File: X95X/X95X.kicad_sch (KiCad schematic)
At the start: 21 parts, among them J1 AVR-ISP-6, J2 USB_C_Receptacle_USB2.0, SW92 SW_Push, U1 ATmega32U4-A, Y1 Crystal_GND24_Small

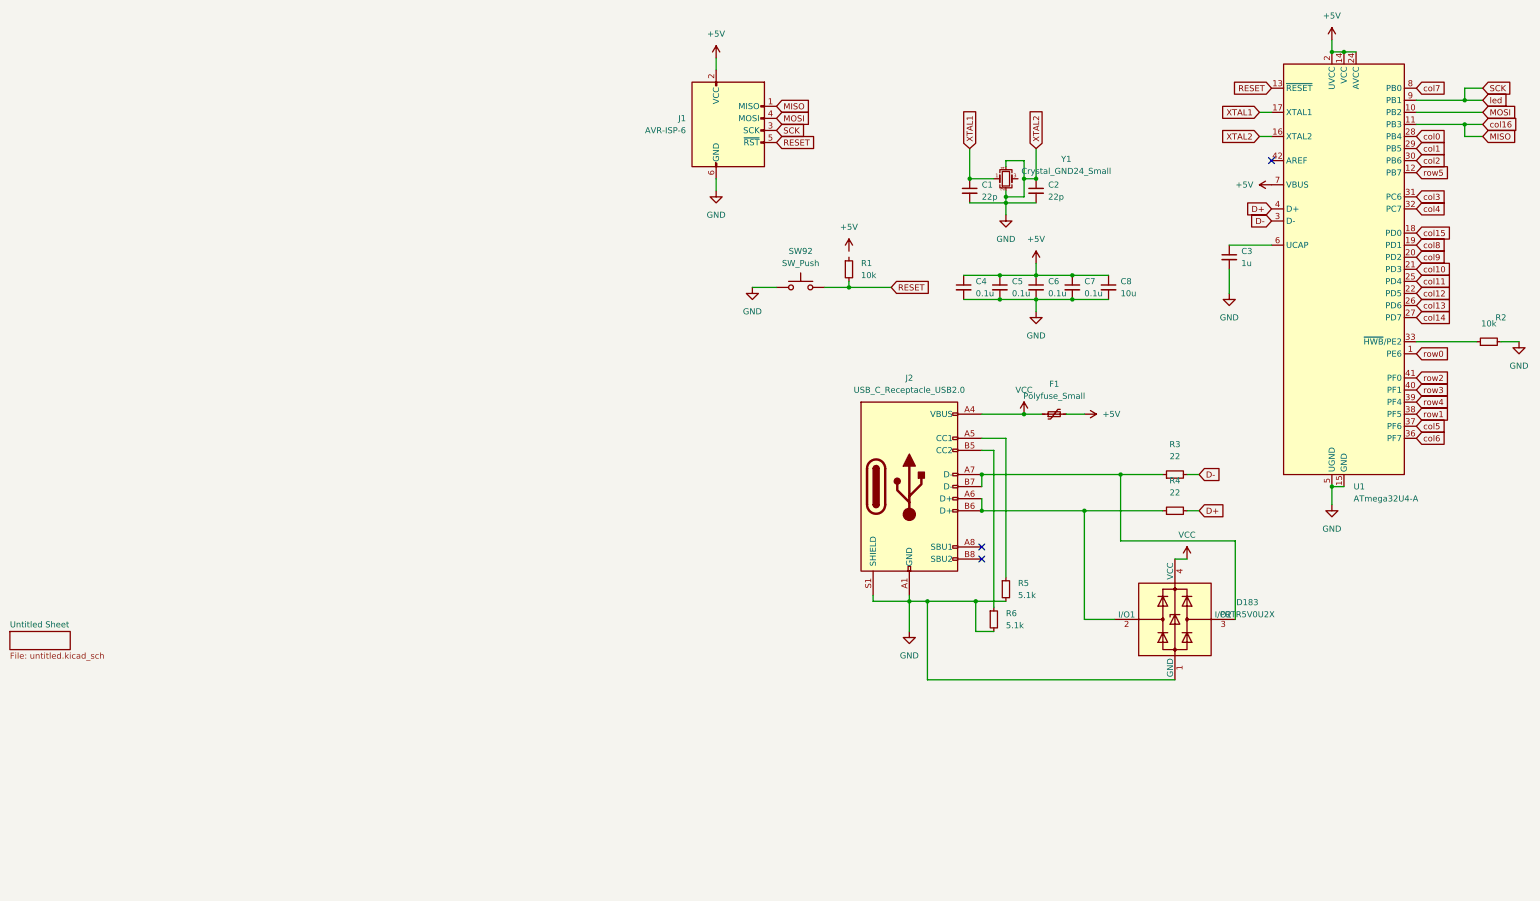
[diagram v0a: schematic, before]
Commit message: v1za
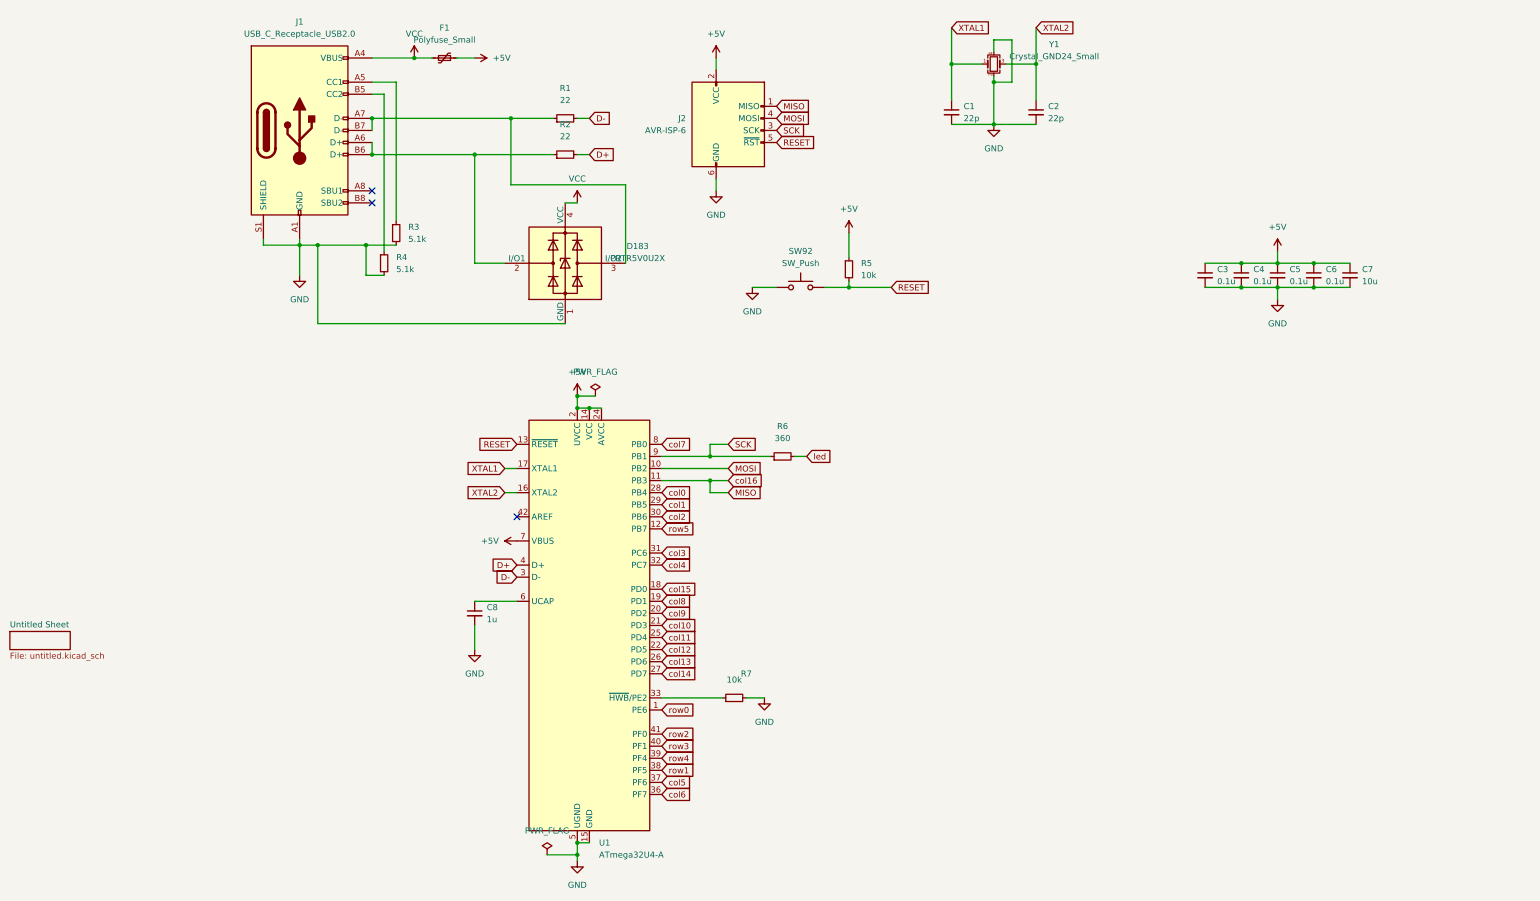
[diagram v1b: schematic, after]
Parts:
- added R6: 360, symbol Device:R_Small
- renumbered C4 to C3, C5 to C4, C6 to C5, C7 to C6, C8 to C7, C3 to C8, J2 to J1, J1 to J2, R3 to R1, R4 to R2, R5 to R3, R6 to R4, R1 to R5, R2 to R7
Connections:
- net +5V: now also R5.1
- net GND: no longer C2.1, U1.16 (XTAL2)
- net SCK: now also R6.1
- net XTAL2: now reaches Y1.3
- net XTAL2: now also C2.1, U1.16 (XTAL2)
- new net led: R6.2
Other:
- moved on the sheet: C3, C4, C5, C6, C7, C8, D183, F1, J1, R1, R2, R3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

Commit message: v1zac
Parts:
- C1, C2, C3, C4, C5, C6, C7, C8: footprint (none) -> Capacitor_SMD:C_0805_2012Metric_Pad1.18x1.45mm_HandSolder
- F1: footprint (none) -> Fuse:Fuse_1206_3216Metric_Pad1.42x1.75mm_HandSolder

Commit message: PCB!!!
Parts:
- D183: footprint Package_TO_SOT_SMD:SOT-143 -> random-keyboard-parts:SOT143B
- J1: footprint (none) -> marbastlib-various:USB_C_Receptacle_HRO_TYPE-C-31-M-14
- J2: footprint (none) -> random-keyboard-parts:Reset_Pretty-Mask
- R1, R2, R3, R4, R5, R6, R7: footprint (none) -> Resistor_SMD:R_0805_2012Metric_Pad1.20x1.40mm_HandSolder
- SW92: footprint (none) -> marbastlib-various:SW_SPST_SKQG_WithStem
- Y1: footprint (none) -> Crystal:Crystal_SMD_3225-4Pin_3.2x2.5mm_HandSoldering
